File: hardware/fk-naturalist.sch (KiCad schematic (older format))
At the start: 132 parts, among them J1 Conn_01x08, J10 S2B-PH-SM4-TB, J11 RF-SMA-EDGE, J2 Conn_01x08, J5 Conn_01x03, J6 Conn_01x05, J7 CONN-HDR-2x5, J8 Conn_01x09, J9 MICRO-USB, M1 MOUNT_HOLE, M3 MOUNT_HOLE, M4 MOUNT_HOLE, M6 MOUNT_HOLE, M7 MICROSD, Q1 2N7002LT1G, Q2 2N7002LT1G, Q3 2N7002LT1G, Q4 2N7002LT1G, SW1 SPNO, SW2 SPNO, U1 ATWINC1500-MR210PA, U10 FGPMMOPA6H, U101 TSL2591, U102 MPL3115A2, U103 BNO055, U104 SHT31, U11 MAX1704XX, U2 ATSAMD21G18A-AU, U3 SPH0645, U4 24AA02E64, U5 S25FL116K0XMFI041, U6 BQ24074RGTT, U7 PCF8523, U8 MCP1700T-3302E/MB, U9 ISL8541x, Y1 FC-135, Y101 FC-135, Y2 FC-135

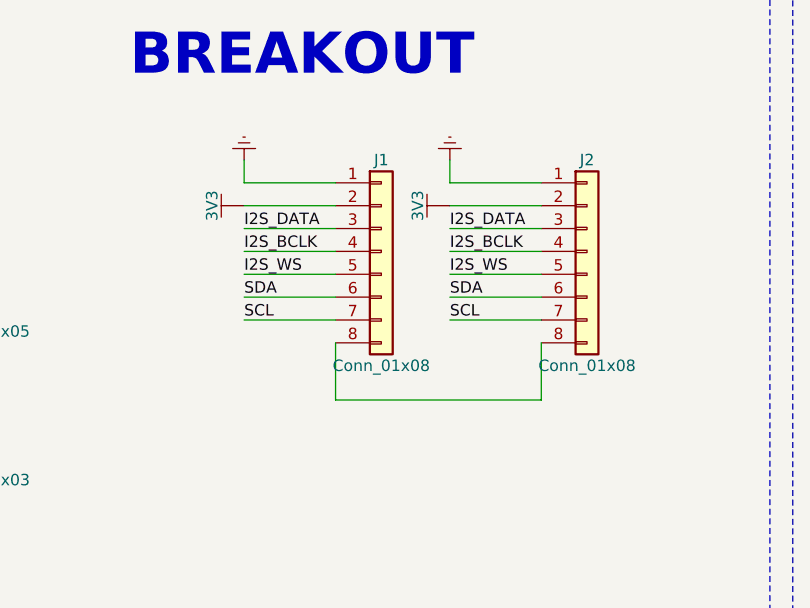
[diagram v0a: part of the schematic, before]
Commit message: New breakaway approach. Cleaning some things up.
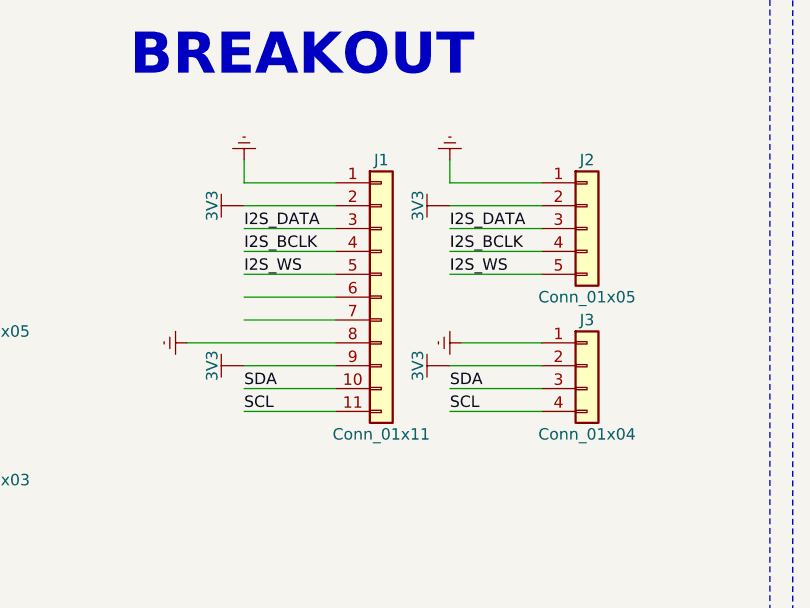
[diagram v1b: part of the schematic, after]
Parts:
- removed J1, J2: Conn_01x08, Socket_Strips:Socket_Strip_Straight_1x08_Pitch2.54mm, symbol Conn_01x08
- added J1: Conn_01x11, Socket_Strips:Socket_Strip_Straight_1x11_Pitch2.54mm, symbol Conn_01x11
- added J2: Conn_01x05, Socket_Strips:Socket_Strip_Straight_1x05_Pitch2.54mm, symbol Conn_01x05
- added J3: Conn_01x04, Socket_Strips:Socket_Strip_Straight_1x04_Pitch2.54mm, symbol Conn_01x04
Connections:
- wire segments 485 -> 488
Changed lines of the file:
@@
 Wire Wire Line
 	900  2800 900  2950
-Text Label 2700 9600 0    50   ~ 0
+Text Label 2700 10000 0    50   ~ 0
 SDA
-Text Label 2700 9700 0    50   ~ 0
+Text Label 2700 10100 0    50   ~ 0
 SCL
 $Comp
@@
 Wire Wire Line
 	2700 9700 3100 9700
-Text Label 3600 9600 0    50   ~ 0
+Text Label 3600 10000 0    50   ~ 0
 SDA
-Text Label 3600 9700 0    50   ~ 0
+Text Label 3600 10100 0    50   ~ 0
 SCL
 $Comp
@@
 Text Label 3600 9500 0    50   ~ 0
 I2S_WS
-$Comp
-L Conn_01x08 J2
-U 1 1 5A5E9723
-P 4200 9400
-F 0 "J2" H 4200 9800 50  0000 C CNN
-F 1 "Conn_01x08" H 4200 8900 50  0000 C CNN
-F 2 "Socket_Strips:Socket_Strip_Straight_1x08_Pitch2.54mm" H 4200 9400 50  0001 C CNN
-F 3 "" H 4200 9400 50  0001 C CNN
-	1    4200 9400
-	1    0    0    -1
-$EndComp
 Wire Wire Line
 	4000 9100 3600 9100
@@
 Wire Wire Line
 	3600 9500 4000 9500
-Wire Wire Line
-	3600 9600 4000 9600
-Wire Wire Line
-	3600 9700 4000 9700
 $Comp
-L Conn_01x08 J1
-U 1 1 5A5DE4BD
-P 3300 9400
-F 0 "J1" H 3300 9800 50  0000 C CNN
-F 1 "Conn_01x08" H 3300 8900 50  0000 C CNN
-F 2 "Socket_Strips:Socket_Strip_Straight_1x08_Pitch2.54mm" H 3300 9400 50  0001 C CNN
-F 3 "" H 3300 9400 50  0001 C CNN
-	1    3300 9400
+L Conn_01x11 J1
+U 1 1 5A5EA7E8
+P 3300 9600
+F 0 "J1" H 3300 10200 50  0000 C CNN
+F 1 "Conn_01x11" H 3300 9000 50  0000 C CNN
+F 2 "Socket_Strips:Socket_Strip_Straight_1x11_Pitch2.54mm" H 3300 9600 50  0001 C CNN
+F 3 "" H 3300 9600 50  0001 C CNN
+	1    3300 9600
 	1    0    0    -1
 $EndComp
+$Comp
+L 3V3 #PWR0117
+U 1 1 5A5EB2B4
+P 2700 9900
+F 0 "#PWR0117" H 2700 9750 50  0001 C CNN
+F 1 "3V3" H 2700 10040 50  0000 C CNN
+F 2 "" H 2700 9900 60  0000 C CNN
+F 3 "" H 2700 9900 60  0000 C CNN
+	1    2700 9900
+	0    -1   -1   0
+$EndComp
+$Comp
+L GND #PWR0118
+U 1 1 5A5EB448
+P 2450 9800
+F 0 "#PWR0118" H 2450 9550 50  0001 C CNN
+F 1 "GND" H 2450 9650 50  0001 C CNN
+F 2 "" H 2450 9800 60  0000 C CNN
+F 3 "" H 2450 9800 60  0000 C CNN
+	1    2450 9800
+	0    1    1    0
+$EndComp
 Wire Wire Line
-	4000 9800 4000 10050
+	2450 9800 3100 9800
 Wire Wire Line
-	4000 10050 3100 10050
+	2700 9900 3100 9900
 Wire Wire Line
-	3100 10050 3100 9800
+	2700 10000 3100 10000
+Wire Wire Line
+	2700 10100 3100 10100
+$Comp
+L 3V3 #PWR0119
+U 1 1 5A5EC9F7
+P 3600 9900
+F 0 "#PWR0119" H 3600 9750 50  0001 C CNN
+F 1 "3V3" H 3600 10040 50  0000 C CNN
+F 2 "" H 3600 9900 60  0000 C CNN
+F 3 "" H 3600 9900 60  0000 C CNN
+	1    3600 9900
+	0    -1   -1   0
+$EndComp
+$Comp
+L GND #PWR0120
+U 1 1 5A5ECB8B
+P 3650 9800
+F 0 "#PWR0120" H 3650 9550 50  0001 C CNN
+F 1 "GND" H 3650 9650 50  0001 C CNN
+F 2 "" H 3650 9800 60  0000 C CNN
+F 3 "" H 3650 9800 60  0000 C CNN
+	1    3650 9800
+	0    1    1    0
+$EndComp
+Wire Wire Line
+	3600 9900 4000 9900
+Wire Wire Line
+	4000 9800 3650 9800
+Wire Wire Line
+	3600 10000 4000 10000
+Wire Wire Line
+	4000 10100 3600 10100
+$Comp
+L Conn_01x05 J2
+U 1 1 5A5F2A47
+P 4200 9300
+F 0 "J2" H 4200 9600 50  0000 C CNN
+F 1 "Conn_01x05" H 4200 9000 50  0000 C CNN
+F 2 "Socket_Strips:Socket_Strip_Straight_1x05_Pitch2.54mm" H 4200 9300 50  0001 C CNN
+F 3 "" H 4200 9300 50  0001 C CNN
+	1    4200 9300
+	1    0    0    -1
+$EndComp
+$Comp
+L Conn_01x04 J3
+U 1 1 5A5F2C0D
+P 4200 9900
+F 0 "J3" H 4200 10100 50  0000 C CNN
+F 1 "Conn_01x04" H 4200 9600 50  0000 C CNN
+F 2 "Socket_Strips:Socket_Strip_Straight_1x04_Pitch2.54mm" H 4200 9900 50  0001 C CNN
+F 3 "" H 4200 9900 50  0001 C CNN
+	1    4200 9900
+	1    0    0    -1
+$EndComp
 $EndSCHEMATC
